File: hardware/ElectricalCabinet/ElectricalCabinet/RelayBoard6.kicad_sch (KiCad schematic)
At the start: 0 parts

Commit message: Further wiring updates
Populated 6100 Bus
Corrected number of relay boards
Added 110v outputs to relay boards and noted light positon
Uploaded light scheme to documents folder
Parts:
- added C6: 0.1uF, Capacitor_SMD:C_0805_2012Metric, symbol Device:C
- added D41, D42, D43, D44, D45, D46, D47, D48: LED, LED_SMD:LED_0805_2012Metric, symbol Device:LED
- added J12: Screw_Terminal_01x06, TerminalBlock:TerminalBlock_MaiXu_MX126-5.0-06P_1x06_P5.00mm, symbol Connector:Screw_Terminal_01x06
- added J13: Screw_Terminal_01x09, TerminalBlock:TerminalBlock_MaiXu_MX126-5.0-09P_1x09_P5.00mm, symbol Connector:Screw_Terminal_01x09
- added K41, K42, K43, K44, K45, K46, K47, K48: G3MB-202P DC5, TrafficLightLibrary:G3MB_202P_DC5, symbol TrafficLightLibrary:G3MB-202P_DC5
- added R41, R42, R43, R44, R45, R46, R47, R48: 1kΩ, Resistor_SMD:R_0805_2012Metric, symbol Device:R
- added U7: TPIC6B595N, TrafficLightLibrary:TPIC6B595N, symbol TrafficLightLibrary:TPIC6B595N
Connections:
- new net: D48.1 (K), R48.1
- new net: D41.2 (A), D42.2 (A), D43.2 (A), D44.2 (A), D45.2 (A), D46.2 (A), D47.2 (A), D48.2 (A), K41.3, K42.3, K43.3, K44.3, K45.3, K46.3, K47.3, K48.3
- new net: D45.1 (K), R45.1
- new net: K45.4, R45.2, U7.14 (DRAIN4)
- new net: D47.1 (K), R47.1
- new net: D42.1 (K), R42.1
- new net: K42.4, R42.2, U7.5 (DRAIN1)
- new net: J13.9 (Pin_9), K41.1, K42.1, K43.1, K44.1, K45.1, K46.1, K47.1, K48.1
- new net: J13.5 (Pin_5), K45.2
- new net: D44.1 (K), R44.1
- new net: C6.1, J12.2 (Pin_2), U7.10 (GND), U7.11 (GND), U7.19 (GND), U7.9 (~{G})
- new net: J12.4 (Pin_4), U7.12 (RCK)
- new net: J12.3 (Pin_3), U7.13 (SRCK)
- new net: K46.4, R46.2, U7.15 (DRAIN5)
- new net: K47.4, R47.2, U7.16 (DRAIN6)
- new net: K48.4, R48.2, U7.17 (DRAIN7)
- new net: J12.1 (Pin_1), U7.18 (SEROUT)
- new net: C6.2, J12.6 (Pin_6), U7.2 (VCC), U7.8 (~{SRCLR})
- new net: K41.4, R41.2, U7.4 (DRAIN0)
- new net: K43.4, R43.2, U7.6 (DRAIN2)
- new net: K44.4, R44.2, U7.7 (DRAIN3)
- new net: D43.1 (K), R43.1
- new net: D41.1 (K), R41.1
- new net: J13.8 (Pin_8), K48.2
- new net: J13.6 (Pin_6), K46.2
- new net: J13.1 (Pin_1), K41.2
- new net: D46.1 (K), R46.1
- new net: J13.2 (Pin_2), K42.2
- new net: J13.3 (Pin_3), K43.2
- new net: J13.4 (Pin_4), K44.2
- new net: J13.7 (Pin_7), K47.2
- new net SERIN: J12.5 (Pin_5), U7.3 (SERIN)
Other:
- note added: "RELAY MODULE 6"

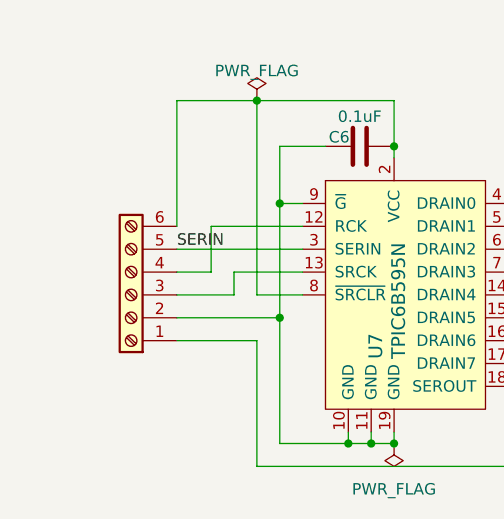
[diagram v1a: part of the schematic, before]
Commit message: Electrical Cabinet done
Electrical Cabinet done, let me know if there are any changes or mistakes.
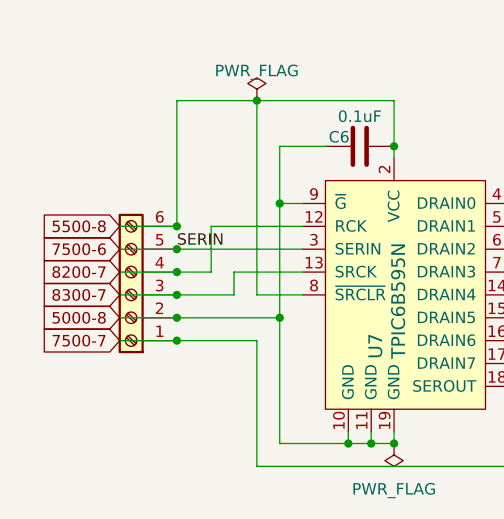
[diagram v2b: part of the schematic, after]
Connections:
- net 5000-8: now reaches C6.1, J12.2 (Pin_2), U7.10 (GND), U7.11 (GND), U7.19 (GND), U7.9 (~{G})
- net 8200-7: now reaches J12.4 (Pin_4), U7.12 (RCK)
- net 8300-7: now reaches J12.3 (Pin_3), U7.13 (SRCK)
- net 7500-7: now reaches J12.1 (Pin_1), U7.18 (SEROUT)
- net 5500-8: now reaches C6.2, J12.6 (Pin_6), U7.2 (VCC), U7.8 (~{SRCLR})
- net SERIN renamed 7500-6
